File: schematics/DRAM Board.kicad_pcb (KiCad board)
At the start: 2 copper layers, 114.3 x 53.3 mm, 17 parts, among them U1 AS4C256K16E0, U16 44256_DRAM, U17 44256_DRAM, U18 44256_DRAM, U19 44256_DRAM, U2 AS4C256K16E0, U20 44256_DRAM, U21 44256_DRAM, U22 44256_DRAM, U23 44256_DRAM, U3 AS4C256K16E0, U4 AS4C256K16E0, U5 LM1117-3.3

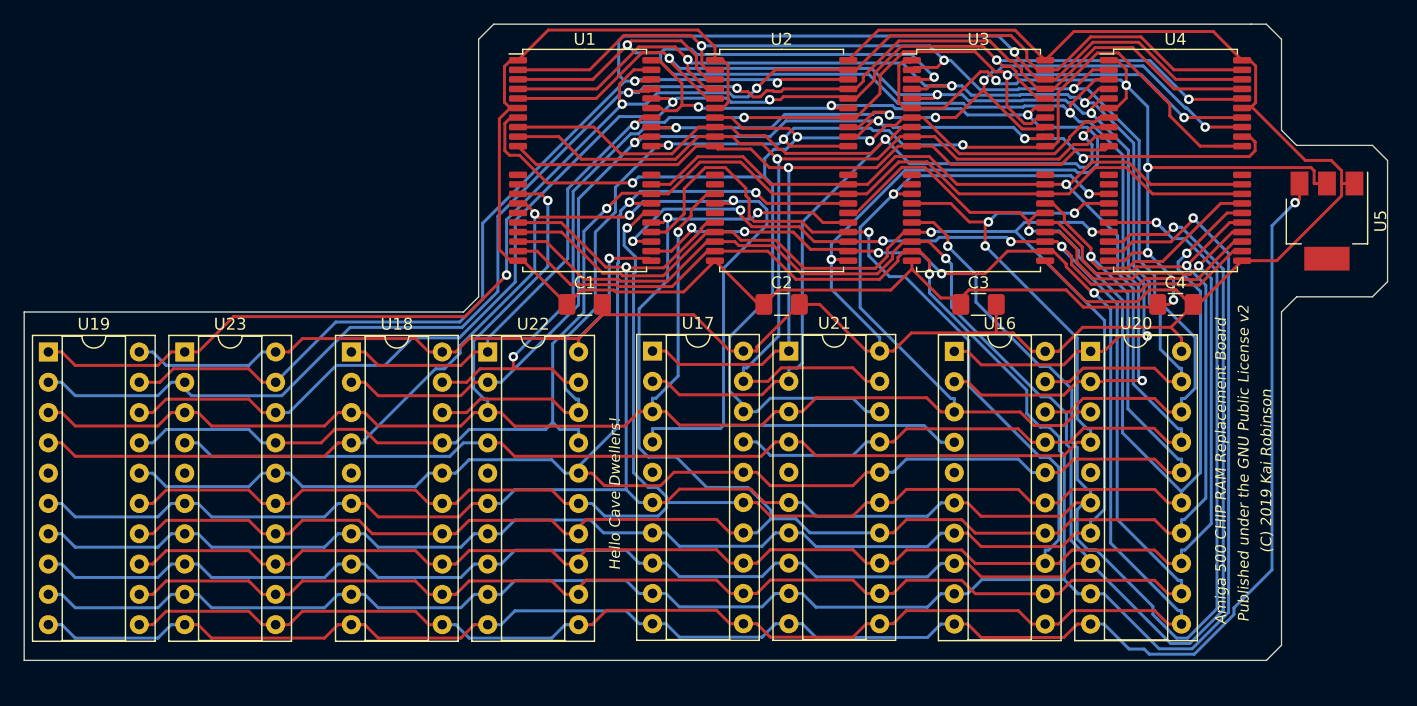
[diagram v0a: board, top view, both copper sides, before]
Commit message: Add files via upload
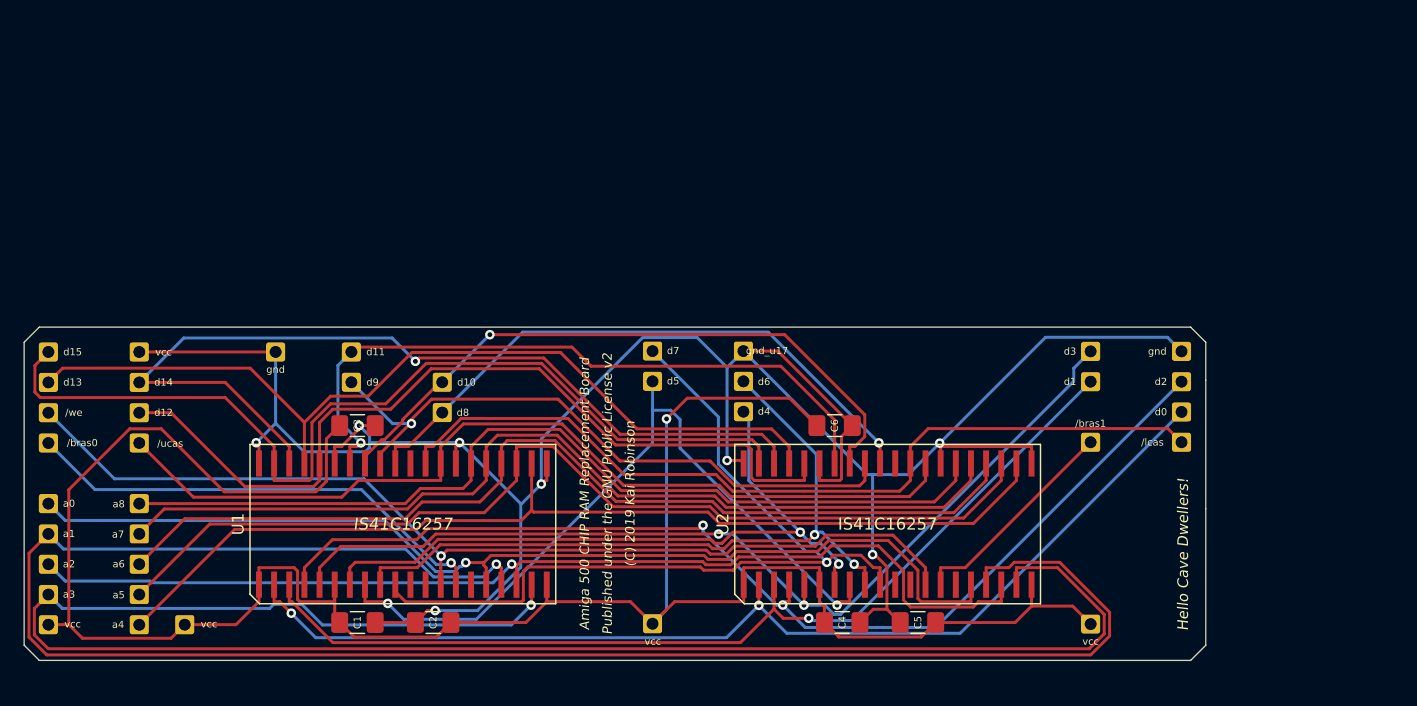
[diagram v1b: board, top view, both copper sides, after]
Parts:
- removed U16, U17, U18, U19, U20, U21, U22, U23: 44256_DRAM, Package_DIP:DIP-20_W7.62mm_Socket
- removed U3, U4: AS4C256K16E0, Package_SO:TSOP-II-40-44_10.16x18.41mm_P0.8mm
- removed U5: LM1117-3.3, Package_TO_SOT_SMD:SOT-223
- added /bras0: Conn_01x01, Connector_PinHeader_2.54mm:PinHeader_1x01_P2.54mm_Vertical, F.Cu at (143.0, 82.1)
- added /bras1: Conn_01x01, Connector_PinHeader_2.54mm:PinHeader_1x01_P2.54mm_Vertical, F.Cu at (230.4, 82.0)
- added /lcas: Conn_01x01, Connector_PinHeader_2.54mm:PinHeader_1x01_P2.54mm_Vertical, F.Cu at (238.0, 82.0)
- added /ucas: Conn_01x01, Connector_PinHeader_2.54mm:PinHeader_1x01_P2.54mm_Vertical, F.Cu at (150.6, 82.1)
- added /we: Conn_01x01, Connector_PinHeader_2.54mm:PinHeader_1x01_P2.54mm_Vertical, F.Cu at (143.0, 79.6)
- added C5: 0.1uF, Capacitor_SMD:C_1206_3216Metric_Pad1.42x1.75mm_HandSolder, F.Cu at (215.9, 97.2)
- added C6: 0.1uF, Capacitor_SMD:C_1206_3216Metric_Pad1.42x1.75mm_HandSolder, F.Cu at (208.9, 80.6)
- added a0: Conn_01x01, Connector_PinHeader_2.54mm:PinHeader_1x01_P2.54mm_Vertical, F.Cu at (143.0, 87.2)
- added a1: Conn_01x01, Connector_PinHeader_2.54mm:PinHeader_1x01_P2.54mm_Vertical, F.Cu at (143.0, 89.7)
- added a2: Conn_01x01, Connector_PinHeader_2.54mm:PinHeader_1x01_P2.54mm_Vertical, F.Cu at (143.0, 92.3)
- added a3: Conn_01x01, Connector_PinHeader_2.54mm:PinHeader_1x01_P2.54mm_Vertical, F.Cu at (143.0, 94.8)
- added a4: Conn_01x01, Connector_PinHeader_2.54mm:PinHeader_1x01_P2.54mm_Vertical, F.Cu at (150.6, 97.3)
- added a5: Conn_01x01, Connector_PinHeader_2.54mm:PinHeader_1x01_P2.54mm_Vertical, F.Cu at (150.6, 94.8)
- added a6: Conn_01x01, Connector_PinHeader_2.54mm:PinHeader_1x01_P2.54mm_Vertical, F.Cu at (150.6, 92.3)
- added a7: Conn_01x01, Connector_PinHeader_2.54mm:PinHeader_1x01_P2.54mm_Vertical, F.Cu at (150.6, 89.7)
- added a8: Conn_01x01, Connector_PinHeader_2.54mm:PinHeader_1x01_P2.54mm_Vertical, F.Cu at (150.6, 87.2)
- added d0: Conn_01x01, Connector_PinHeader_2.54mm:PinHeader_1x01_P2.54mm_Vertical, F.Cu at (238.0, 79.5)
- added d1: Conn_01x01, Connector_PinHeader_2.54mm:PinHeader_1x01_P2.54mm_Vertical, F.Cu at (230.4, 77.0)
- added d10: Conn_01x01, Connector_PinHeader_2.54mm:PinHeader_1x01_P2.54mm_Vertical, F.Cu at (176.0, 77.0)
- added d11: Conn_01x01, Connector_PinHeader_2.54mm:PinHeader_1x01_P2.54mm_Vertical, F.Cu at (168.4, 74.5)
- added d12: Conn_01x01, Connector_PinHeader_2.54mm:PinHeader_1x01_P2.54mm_Vertical, F.Cu at (150.6, 79.6)
- added d13: Conn_01x01, Connector_PinHeader_2.54mm:PinHeader_1x01_P2.54mm_Vertical, F.Cu at (143.0, 77.0)
- added d14: Conn_01x01, Connector_PinHeader_2.54mm:PinHeader_1x01_P2.54mm_Vertical, F.Cu at (150.6, 77.0)
- added d15: Conn_01x01, Connector_PinHeader_2.54mm:PinHeader_1x01_P2.54mm_Vertical, F.Cu at (143.0, 74.5)
- added d2: Conn_01x01, Connector_PinHeader_2.54mm:PinHeader_1x01_P2.54mm_Vertical, F.Cu at (238.0, 77.0)
- added d3: Conn_01x01, Connector_PinHeader_2.54mm:PinHeader_1x01_P2.54mm_Vertical, F.Cu at (230.4, 74.4)
- added d4: Conn_01x01, Connector_PinHeader_2.54mm:PinHeader_1x01_P2.54mm_Vertical, F.Cu at (201.3, 79.5)
- added d5: Conn_01x01, Connector_PinHeader_2.54mm:PinHeader_1x01_P2.54mm_Vertical, F.Cu at (193.7, 76.9)
- added d6: Conn_01x01, Connector_PinHeader_2.54mm:PinHeader_1x01_P2.54mm_Vertical, F.Cu at (201.3, 76.9)
- added d7: Conn_01x01, Connector_PinHeader_2.54mm:PinHeader_1x01_P2.54mm_Vertical, F.Cu at (193.7, 74.4)
- added d8: Conn_01x01, Connector_PinHeader_2.54mm:PinHeader_1x01_P2.54mm_Vertical, F.Cu at (176.0, 79.6)
- added d9: Conn_01x01, Connector_PinHeader_2.54mm:PinHeader_1x01_P2.54mm_Vertical, F.Cu at (168.4, 77.0)
- added gnd_u17: Conn_01x01, Connector_PinHeader_2.54mm:PinHeader_1x01_P2.54mm_Vertical, F.Cu at (201.3, 74.4)
- added gnd_u19: Conn_01x01, Connector_PinHeader_2.54mm:PinHeader_1x01_P2.54mm_Vertical, F.Cu at (150.6, 74.5)
- added gnd_u20: Conn_01x01, Connector_PinHeader_2.54mm:PinHeader_1x01_P2.54mm_Vertical, F.Cu at (238.0, 74.4)
- added gnd_u23: Conn_01x01, Connector_PinHeader_2.54mm:PinHeader_1x01_P2.54mm_Vertical, F.Cu at (162.1, 74.5)
- added vcc_u17: Conn_01x01, Connector_PinHeader_2.54mm:PinHeader_1x01_P2.54mm_Vertical, F.Cu at (193.7, 97.3)
- added vcc_u19: Conn_01x01, Connector_PinHeader_2.54mm:PinHeader_1x01_P2.54mm_Vertical, F.Cu at (143.0, 97.3)
- added vcc_u20: Conn_01x01, Connector_PinHeader_2.54mm:PinHeader_1x01_P2.54mm_Vertical, F.Cu at (230.4, 97.3)
- added vcc_u23: Conn_01x01, Connector_PinHeader_2.54mm:PinHeader_1x01_P2.54mm_Vertical, F.Cu at (154.4, 97.3)
- U1, U2: value AS4C256K16E0 -> IS41C16257; footprint Package_SO:TSOP-II-40-44_10.16x18.41mm_P0.8mm -> Package_SO_J-Lead:SOJ-40
- moved C3 53.1 mm to (168.9, 80.6)
- moved C2 39.6 mm to (175.3, 97.2), turned to 180 degrees
- moved C4 38.6 mm to (209.6, 97.2)
- moved U1 34.1 mm to (172.7, 88.9)
- moved C1 32.8 mm to (168.9, 97.2)
- moved U2 31.8 mm to (213.4, 88.9)
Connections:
- C1 pad 1: /VCC -> /vcc5
- C2 pad 1: /VCC -> /vcc5
- C3 pad 1: /VCC -> /vcc5
- C4 pad 1: /VCC -> /vcc5
- U1 pad 1: /VCC -> /vcc5
- U1 pad 13: Net-(U1-Pad13) -> /_we
- U1 pad 14: Net-(U1-Pad14) -> /_bras0
- U1 pad 15: /_we -> Net-(U1-Pad15)
- U1 pad 16: /_bras0 -> /a0
- U1 pad 17: Net-(U1-Pad17) -> /a1
- U1 pad 18: /a0 -> /a2
- U1 pad 19: /a1 -> /a3
- U1 pad 20: /a2 -> /vcc5
- U1 pad 21: /a3 -> /gnd
- U1 pad 22: /VCC -> /a4
- U1 pad 23: /gnd -> /a5
- U1 pad 24: /a4 -> /a6
- U1 pad 25: /a5 -> /a7
- U1 pad 26: /a6 -> /a8
- U1 pad 27: /a7 -> /gnd
- U1 pad 28: /a8 -> /_ucas
- U1 pad 29: /_oe -> /_lcas
- U1 pad 30: /_ucas -> Net-(U1-Pad30)
- U1 pad 31: /_lcas -> /d8
- U1 pad 32: Net-(U1-Pad32) -> /d9
- U1 pad 35: /d8 -> /gnd
- U1 pad 36: /d9 -> /d12
- U1 pad 37: /d10 -> /d13
- U1 pad 38: /d11 -> /d14
- U1 pad 39: /gnd -> /d15
- U1 pad 40: /d12 -> /gnd
- U1 pad 6: /VCC -> /vcc5
- U2 pad 1: /VCC -> /vcc5
- U2 pad 13: Net-(U2-Pad13) -> /_we
- U2 pad 14: Net-(U2-Pad14) -> /_bras1
- U2 pad 15: /_we -> Net-(U2-Pad15)
- U2 pad 16: /_bras0 -> /a0
- U2 pad 17: Net-(U2-Pad17) -> /a1
- U2 pad 18: /a0 -> /a2
- U2 pad 19: /a1 -> /a3
- U2 pad 20: /a2 -> /vcc5
- U2 pad 21: /a3 -> /gnd
- U2 pad 22: /VCC -> /a4
- U2 pad 23: /gnd -> /a5
- U2 pad 24: /a4 -> /a6
- U2 pad 25: /a5 -> /a7
- U2 pad 26: /a6 -> /a8
- U2 pad 27: /a7 -> /gnd
- U2 pad 28: /a8 -> /_ucas
- U2 pad 29: /_oe -> /_lcas
- U2 pad 30: /_ucas -> Net-(U2-Pad30)
- U2 pad 31: /_lcas -> /d8
- U2 pad 32: Net-(U2-Pad32) -> /d9
- U2 pad 35: /d8 -> /gnd
- U2 pad 36: /d9 -> /d12
- U2 pad 37: /d10 -> /d13
- U2 pad 38: /d11 -> /d14
- U2 pad 39: /gnd -> /d15
- U2 pad 40: /d12 -> /gnd
- U2 pad 6: /VCC -> /vcc5
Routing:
- net /_oe: track 182.9 -> 0.00 mm, vias 3 -> 0
- net /VCC: track 180.0 -> 0.00 mm, vias 5 -> 0
- net /a0: track 223.4 -> 87.9 mm, vias 3 -> 1
- net /a2: track 222.0 -> 88.9 mm, vias 2 -> 1
- net /a8: track 200.2 -> 77.4 mm, vias 3 -> 0
- net /a6: track 202.9 -> 82.0 mm, vias 2 -> 0
- net /a7: track 190.7 -> 79.7 mm, vias 3 -> 0
- net /a5: track 186.9 -> 84.3 mm, vias 5 -> 0
- net /_bras1: track 118.9 -> 18.4 mm, vias 3 -> 0
- net /_we: track 182.4 -> 84.5 mm, vias 4 -> 1
- net /a4: track 180.9 -> 84.8 mm, vias 5 -> 0
- net /gnd: track 292.2 -> 207.3 mm, vias 5 -> 8
- net /_bras0: track 123.7 -> 40.0 mm, vias 3 -> 1
- net /a3: track 222.6 -> 150.8 mm, vias 2 -> 1
- net /d14: track 136.6 -> 76.4 mm, vias 3 -> 1
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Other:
- board size 114.3 x 53.3 mm -> 99.1 x 27.9 mm
- board text added: "IS41C16257"
- board text added: "gnd"
- board text added: "vcc"
